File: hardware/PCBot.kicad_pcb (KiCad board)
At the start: 4 copper layers, 100 x 70 mm, 105 parts, among them J101 Conn_ST_STDC14, SW101 SW_SPDT, U101 STM32G431CBUx, U102 AMS1117-3.3, U103 LSM6DS3, U104 STSPIN250, U105 STSPIN250, U201 A7105, Y101 Crystal_GND24_DNP, Y102 Q13FC1350000400, Y201 Crystal_GND24_DNP

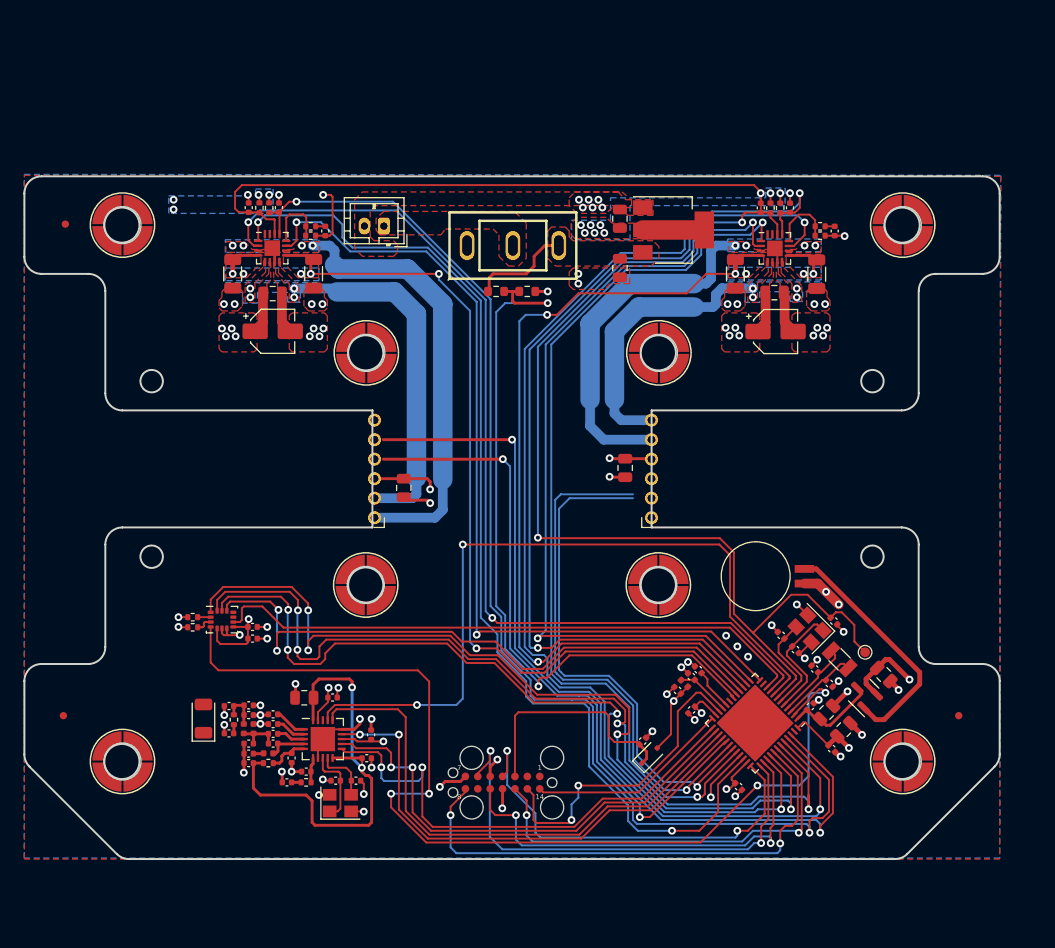
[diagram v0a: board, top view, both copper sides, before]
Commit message: i uhhhhhhhhhhhhhhhhhhhhh
Signed-off-by: Connor Rigby <connorr@hey.com>
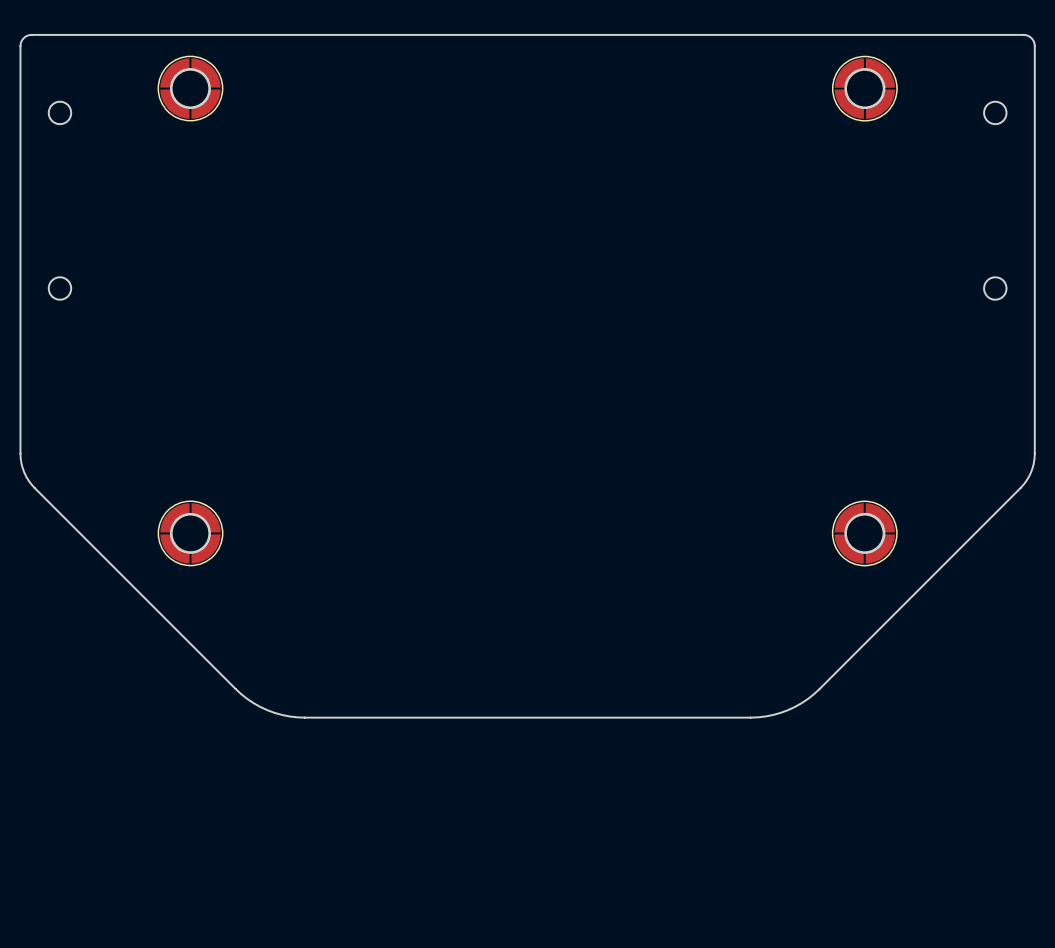
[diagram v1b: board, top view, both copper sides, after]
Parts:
- removed BT101: Battery, Connector_JST:JST_PH_B2B-PH-K_1x02_P2.00mm_Vertical
- removed BT102: Battery_Cell, Battery:BatteryHolder_Seiko_MS621F
- removed C101, C102, C103, C104, C109, C110, C111, C114, C127, C128, C203, C206, C207, C208, C209, C211, C214, C215, C216, C217, C218, C219, C220: C_0402_DNP, Capacitor_SMD:C_0402_1005Metric
- removed C105, C112, C201: C_805_DNP, Capacitor_SMD:C_0805_2012Metric
- removed C106, C113: 22uf, Capacitor_SMD:CP_Elec_4x5.4
- removed C107, C131, C132: C_0805_1u_X7R, Capacitor_SMD:C_0805_2012Metric
- removed C108: C_0805_10u_X5R, Capacitor_SMD:C_0805_2012Metric
- removed C115, C116, C117, C118, C119, C122, C123, C124, C125, C126, C205: C_0402_100nf_X7R, Capacitor_SMD:C_0402_1005Metric
- removed C120, C129, C130: C_0805_4u7_X5R, Capacitor_SMD:C_0805_2012Metric
- removed C121: C_0402_1u_X5R, Capacitor_SMD:C_0402_1005Metric
- removed C202, C204: C_0402_2u2_X5R, Capacitor_SMD:C_0402_1005Metric
- removed C210: C_0402_22p_C0G, Capacitor_SMD:C_0402_1005Metric
- removed C212: C_0402_100p_C0G, Capacitor_SMD:C_0402_1005Metric
- removed C213: C_0402_10n_C0G, Capacitor_SMD:C_0402_1005Metric
- removed D101: 30v 230mv@100ma 1A, Diode_SMD:D_SOD-323F
- removed D106: BAT54C, Package_TO_SOT_SMD:SOT-23
- removed FB101: FerriteBead_Small, Inductor_SMD:L_0402_1005Metric
- removed H101, H102, H103, H104, H105, H106, H107, H108: MountingHole_Pad, LCSC_Connector:SMD_BD5.6-L5.6-W5.6-D3.6
- removed J101: Conn_ST_STDC14, LCSC_Connector:TC2070-IDC-FP
- removed JM1: JM1, Connector_PinHeader_2.00mm:PinHeader_1x06_P2.00mm_Horizontal
- removed JM2: JM2, Connector_PinHeader_2.00mm:PinHeader_1x06_P2.00mm_Horizontal
- removed L202, L203, L204: L_0402_DNP, Inductor_SMD:L_0402_1005Metric
- removed R101, R103, R106, R110: 18k, Resistor_SMD:R_0402_1005Metric
- removed R102, R107: 39k, Resistor_SMD:R_0402_1005Metric
- removed R104, R109, R113, R114: R_0402_1k, Resistor_SMD:R_0402_1005Metric
- removed R105, R108, R115, R116: R_1206_DNP, Resistor_SMD:R_1206_3216Metric
- removed R111, R112: R_0603_DNP, Resistor_SMD:R_0603_1608Metric
- removed R201, R203: DNP, Resistor_SMD:R_0402_1005Metric
- removed R202: 200, Resistor_SMD:R_0402_1005Metric
- removed the REF** at (124.0, 89.4)
- removed the REF** at (32.2, 89.4)
- removed the REF** at (32.4, 39.0)
- removed the REF** at (46.6, 89.7)
- removed SW101: SW_SPDT, LCSC_Switch:SW-TH_SS-12D16L3R
- removed TP101: RESET, TestPoint:TestPoint_Pad_D1.0mm
- removed U101: STM32G431CBUx, Package_DFN_QFN:QFN-48-1EP_7x7mm_P0.5mm_EP5.6x5.6mm
- removed U102: AMS1117-3.3, Package_TO_SOT_SMD:SOT-223-3_TabPin2
- removed U103: LSM6DS3, Package_LGA:LGA-14_3x2.5mm_P0.5mm_LayoutBorder3x4y
- removed U104, U105: STSPIN250, Package_DFN_QFN:TQFN-16-1EP_3x3mm_P0.5mm_EP1.6x1.6mm
- removed U201: A7105, Package_DFN_QFN:QFN-20-1EP_4x4mm_P0.5mm_EP2.5x2.5mm
- removed Y101, Y201: Crystal_GND24_DNP, Crystal:Crystal_SMD_3225-4Pin_3.2x2.5mm
- removed Y102: Q13FC1350000400, Crystal:Crystal_SMD_3215-2Pin_3.2x1.5mm
- added REF**: SMD_BD5.6-L5.6-W5.6-D3.6, LCSC_Connector:SMD_BD5.6-L5.6-W5.6-D3.6, F.Cu at (45.2, 70.7)
- added REF**: SMD_BD5.6-L5.6-W5.6-D3.6, LCSC_Connector:SMD_BD5.6-L5.6-W5.6-D3.6, F.Cu at (114.4, 70.7)
- added REF**: SMD_BD5.6-L5.6-W5.6-D3.6, LCSC_Connector:SMD_BD5.6-L5.6-W5.6-D3.6, F.Cu at (45.2, 25.1)
- added REF**: SMD_BD5.6-L5.6-W5.6-D3.6, LCSC_Connector:SMD_BD5.6-L5.6-W5.6-D3.6, F.Cu at (114.4, 25.1)
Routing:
- net /~{RESET}: track 173.0 -> 0.00 mm, vias 2 -> 0
- net /M2_EN_FAULT: track 124.0 -> 0.00 mm, vias 2 -> 0
- net /M1_EN_FAULT: track 123.3 -> 0.00 mm, vias 2 -> 0
- net /M2_DIR: track 109.1 -> 0.00 mm, vias 2 -> 0
- net /IMU_IRQ1: track 105.3 -> 0.00 mm, vias 4 -> 0
- net /M2_PWM: track 99.0 -> 0.00 mm, vias 2 -> 0
- net GND: track 94.8 -> 0.00 mm, vias 78 -> 0
- net /M1_DIR: track 93.2 -> 0.00 mm, vias 2 -> 0
- net /M1_REF: track 93.1 -> 0.00 mm, vias 2 -> 0
- net /M1_SENSE: track 92.2 -> 0.00 mm, vias 6 -> 0
- net /M2_SENSE: track 92.0 -> 0.00 mm, vias 6 -> 0
- net /SPI3_MOSI: track 92.0 -> 0.00 mm, vias 4 -> 0
- net /M2_REF: track 90.4 -> 0.00 mm, vias 2 -> 0
- net /M2_ENC_N: track 90.1 -> 0.00 mm, vias 2 -> 0
- net /SPI3_MISO: track 88.2 -> 0.00 mm, vias 4 -> 0
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- removed copper zone on F.Cu, net +BATT
- removed copper zone on In2.Cu, net +BATT
- removed copper zone on B.Cu, net /M1_OUTA1
- removed copper zone on F.Cu, net /M1_OUTA1
- removed copper zone on B.Cu, net /M1_OUTA2
- removed copper zone on F.Cu, net /M1_OUTA2
- removed copper zone on B.Cu, net /M1_SENSE
- removed copper zone on F.Cu, net /M1_SENSE
- removed copper zone on B.Cu, net /M2_OUTA1
- removed copper zone on F.Cu, net /M2_OUTA1
- removed copper zone on B.Cu, net /M2_OUTA2
- removed copper zone on F.Cu, net /M2_OUTA2
- removed copper zone on B.Cu, net /M2_SENSE
- removed copper zone on F.Cu, net /M2_SENSE
- removed copper zone on F.Cu, net /VBAT_IN
- removed copper zone on B.Cu, net GND
- removed copper zone on F.Cu, net GND
- removed copper zone on In1.Cu, net GND
- removed copper zone on B.Cu, net VDD
- removed copper zone on F.Cu, net VDD
- removed copper zone on In2.Cu, net VDD
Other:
- board size 100 x 70 mm -> 104 x 70 mm

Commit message: sdfasdfa
Signed-off-by: Connor Rigby <connorr@hey.com>
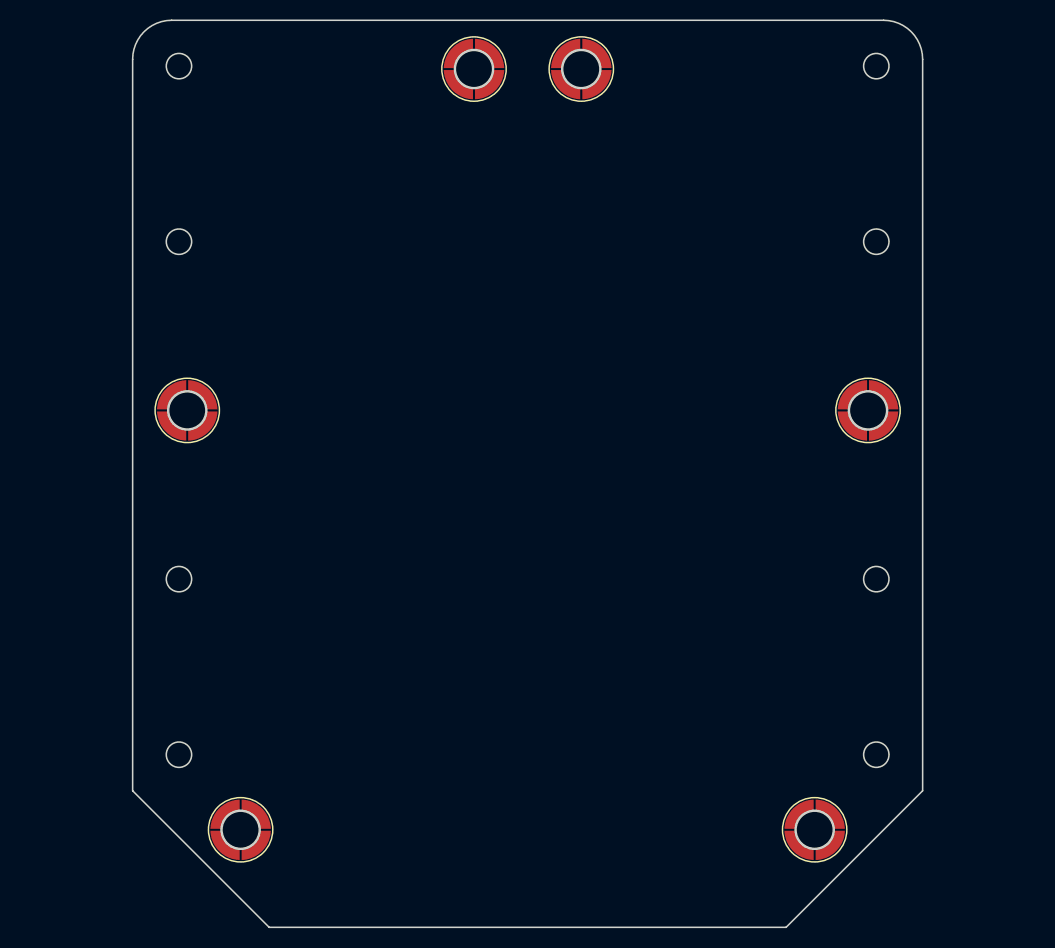
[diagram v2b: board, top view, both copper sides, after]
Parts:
- removed the REF** at (45.2, 70.7)
- removed the REF** at (114.4, 70.7)
- removed the REF** at (45.2, 25.1)
- removed the REF** at (114.4, 25.1)
- added REF**: SMD_BD5.6-L5.6-W5.6-D3.6, LCSC_Connector:SMD_BD5.6-L5.6-W5.6-D3.6, F.Cu at (50.4, 101.1)
- added REF**: SMD_BD5.6-L5.6-W5.6-D3.6, LCSC_Connector:SMD_BD5.6-L5.6-W5.6-D3.6, F.Cu at (85.3, 23.1)
- added REF**: SMD_BD5.6-L5.6-W5.6-D3.6, LCSC_Connector:SMD_BD5.6-L5.6-W5.6-D3.6, F.Cu at (74.3, 23.1)
- added REF**: SMD_BD5.6-L5.6-W5.6-D3.6, LCSC_Connector:SMD_BD5.6-L5.6-W5.6-D3.6, F.Cu at (114.7, 58.1)
- added REF**: SMD_BD5.6-L5.6-W5.6-D3.6, LCSC_Connector:SMD_BD5.6-L5.6-W5.6-D3.6, F.Cu at (44.9, 58.1)
- added REF**: SMD_BD5.6-L5.6-W5.6-D3.6, LCSC_Connector:SMD_BD5.6-L5.6-W5.6-D3.6, F.Cu at (109.2, 101.1)
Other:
- board size 104 x 70 mm -> 81 x 93 mm
